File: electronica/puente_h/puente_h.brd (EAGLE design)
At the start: 100 x 80 mm, 40 parts, among them IC1 7805, IC2 7812, IC3 74HC04N, IC4 74HC08N, IC5 ADUM1400, Q1 IRF2804, Q2 IRF2804, Q5 IRF2804, Q6 IRF2804, U3 IR2110

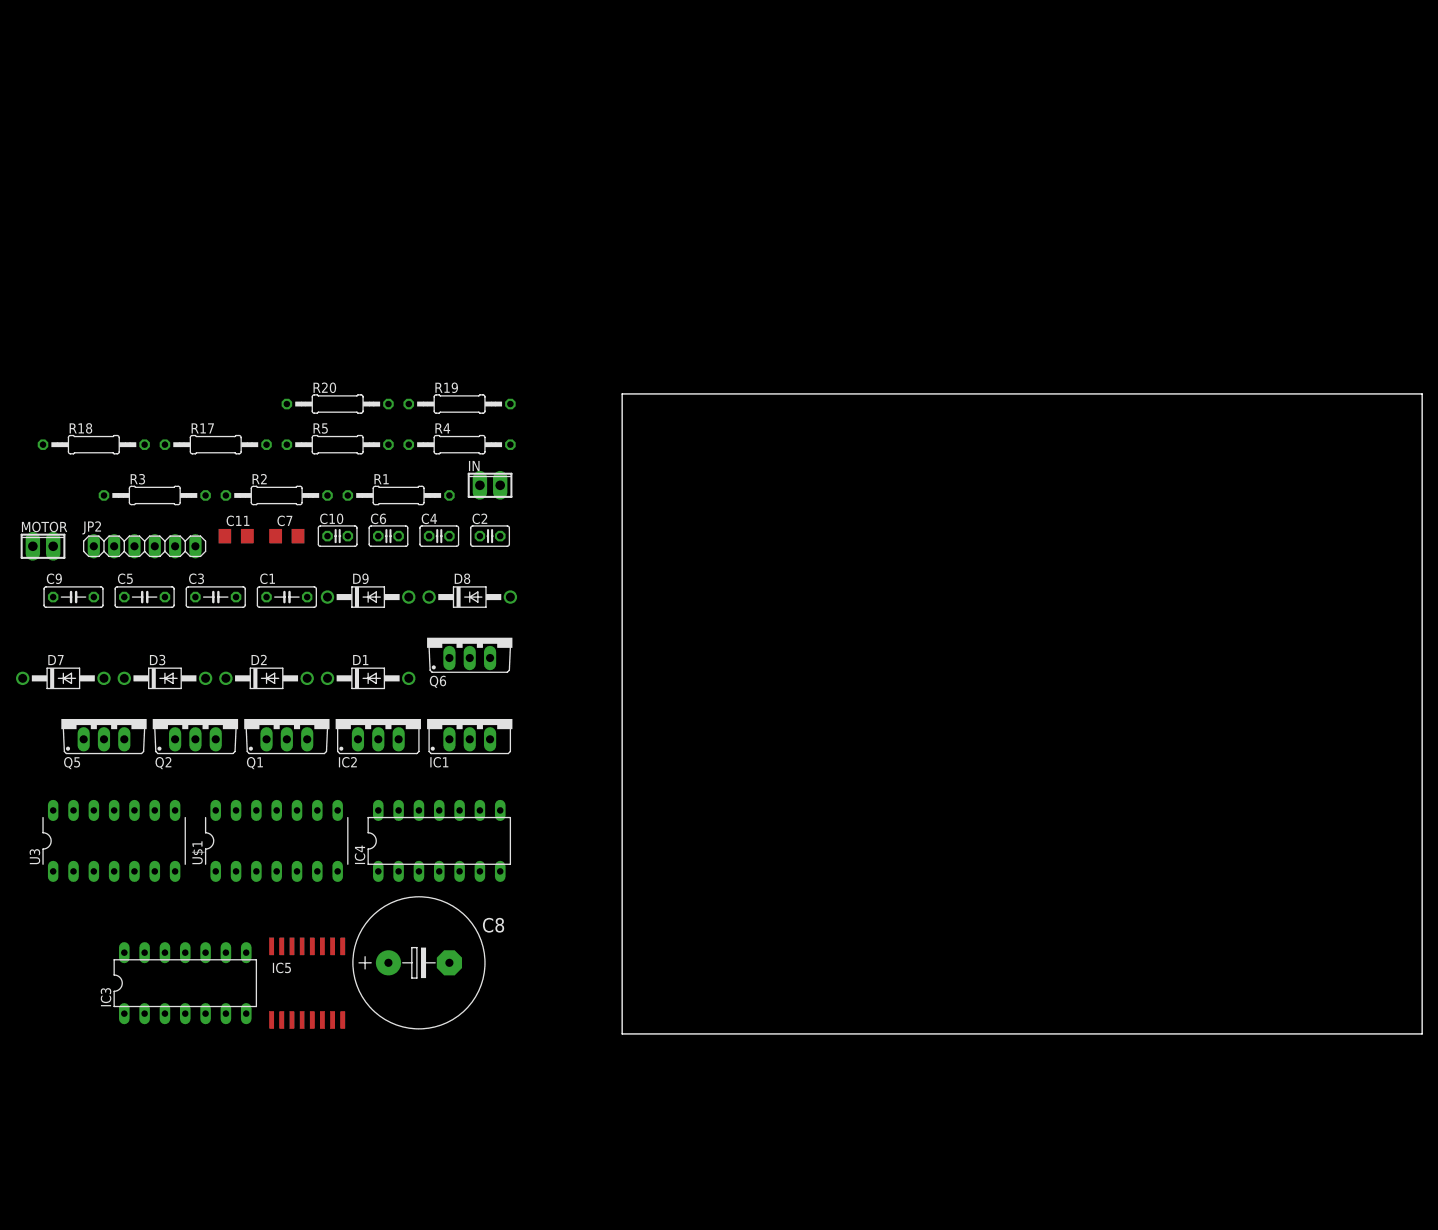
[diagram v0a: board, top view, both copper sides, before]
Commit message: pads mas largos
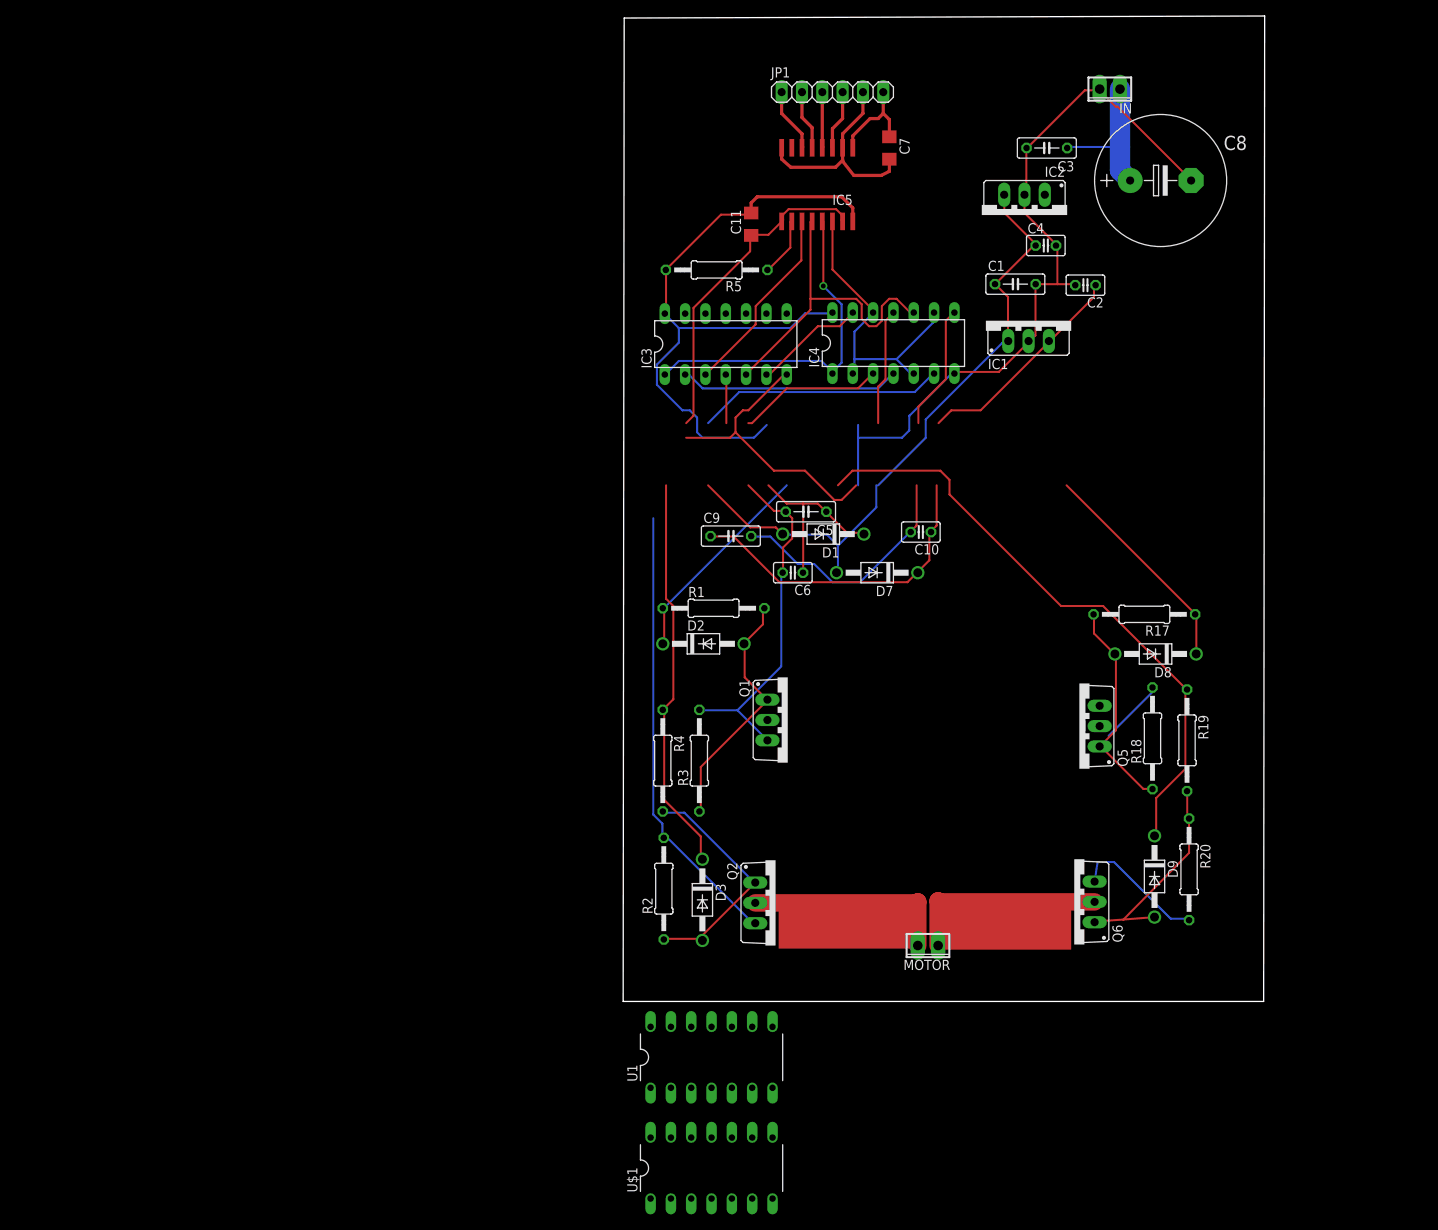
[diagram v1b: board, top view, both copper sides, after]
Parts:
- removed JP2: (no value), pinhead:1X06
- removed U3: IR2110, components:IR2110
- added JP1: (no value), pinhead:1X06
- added U1: IR2110LP, components:IR2110-LP
- U$1: value IR2110 -> IR2110LP; device components:IR2110 -> components:IR2110-LP
- moved R18 137.3 mm to (66.3, 37.0), turned to 90 degrees
- moved C8 134.8 mm to (67.3, 106.7)
- moved Q5 121.9 mm to (57.1, 38.5), turned to 90 degrees
- moved MOTOR 121.4 mm to (38.2, 11.0), turned to 180 degrees
- moved R20 121.3 mm to (70.9, 20.6), turned to 270 degrees
- moved IC5 118.4 mm to (24.4, 106.2), turned to 180 degrees
- moved C3 118.1 mm to (53.1, 110.7), turned to 180 degrees
- moved R17 118.0 mm to (65.3, 52.5), turned to 180 degrees
- moved D9 105.1 mm to (66.5, 21.0), turned to 270 degrees
- moved D7 105.1 mm to (33.1, 57.7), turned to 180 degrees
- moved IC3 104.6 mm to (13.0, 86.2)
- moved IC2 102.4 mm to (50.3, 102.4), turned to 180 degrees
- moved R19 100.2 mm to (70.6, 36.7), turned to 270 degrees
- moved C1 99.1 mm to (49.1, 93.7)
- moved IN 92.0 mm to (61.0, 118.1), turned to 180 degrees
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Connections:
- removed net GND1@2: C7.2, IC5.2, IC5.8, JP2.2
- removed net N$13: IC5.4, JP2.4
- removed net N$14: IC5.5, JP2.5
- removed net N$8: IC5.3, JP2.3
- new net N$20: IC5.6, JP1.1
- new net N$21: IC5.4, JP1.3
- new net N$22: IC5.3, JP1.4
- new net N$24: C7.1, IC5.1, JP1.6
- net +12V: now also U1.3; no longer U3.3
- net +5V: now also U1.9; no longer U3.9
- net GND: now also U1.13, U1.2; no longer U3.13, U3.2
- net N$1: now also U1.6; no longer U$1.6
- net N$11: now also U1.10; no longer U$1.10
- net N$12: now also U1.12; no longer U$1.12
- net N$15: now also IC5.5, JP1.2; no longer IC5.6, JP2.6
- net N$19: now also U$1.12; no longer U3.12
- net N$2: now also U1.7; no longer U$1.7
- net N$3: now also U1.5; no longer U$1.5
- net N$30: now also U$1.6; no longer U3.6
- net N$31: now also U$1.5; no longer U3.5
- net N$32: now also U$1.7; no longer U3.7
- net N$35: now also U$1.1; no longer U3.1
- net N$5: now also C7.2, IC5.2, IC5.8, JP1.5; no longer C7.1, IC5.1, JP2.1
- net N$6: now also U1.1; no longer U$1.1
- net N$9: now also U$1.10; no longer U3.10
- net SD: now also U1.11; no longer U3.11
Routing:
- net GND: track 0.00 -> 246.0 mm
- net +5V: track 0.00 -> 112.4 mm
- net +12V: track 0.00 -> 80.4 mm
- net N$35: track 0.00 -> 76.8 mm
- net N$3: track 0.00 -> 70.1 mm
- net N$31: track 0.00 -> 65.8 mm
- net N$6: track 0.00 -> 49.8 mm
- net A: track 0.00 -> 42.7 mm, vias 0 -> 1
- net B: track 0.00 -> 41.2 mm
- net N$30: track 0.00 -> 40.7 mm
- net EN: track 0.00 -> 38.3 mm
- net N$4: track 0.00 -> 31.2 mm
- net N$12: track 0.00 -> 30.8 mm
- net N$7: track 0.00 -> 30.1 mm
- net N$5: track 0.00 -> 27.8 mm
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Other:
- board size 100 x 80 mm -> 80.2 x 123.2 mm
